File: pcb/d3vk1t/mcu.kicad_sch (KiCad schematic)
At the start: 11 parts, among them J2 Conn_01x06, U1 STM32F412RETx

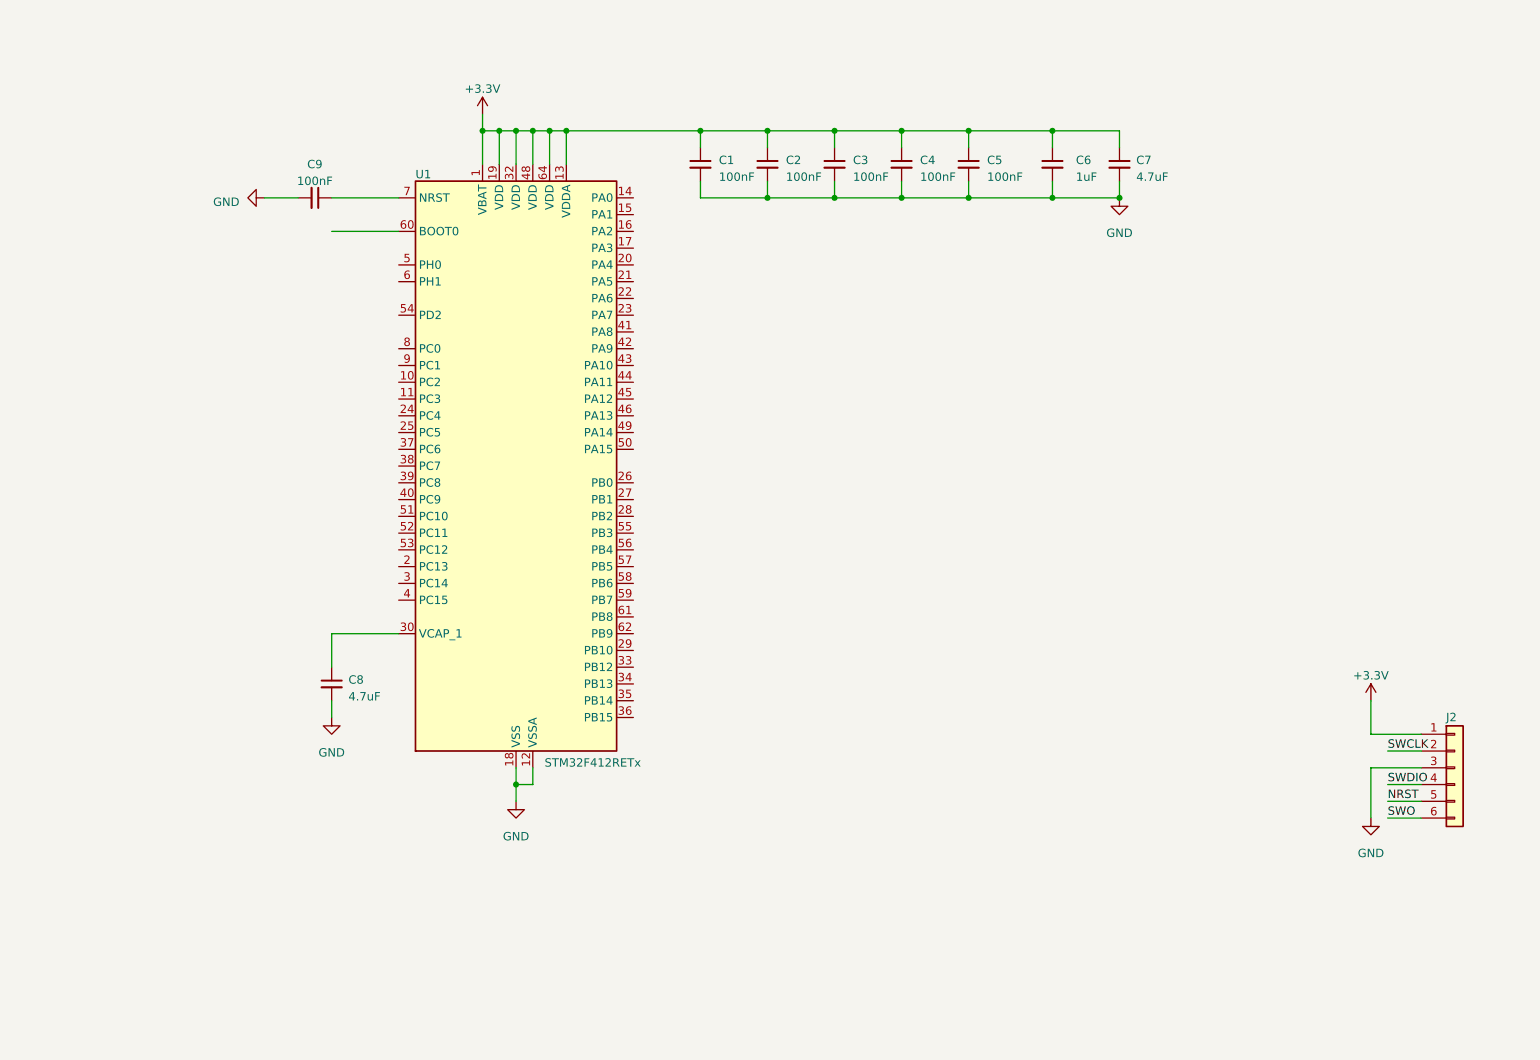
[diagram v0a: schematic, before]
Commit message: [update all schematics sheets]
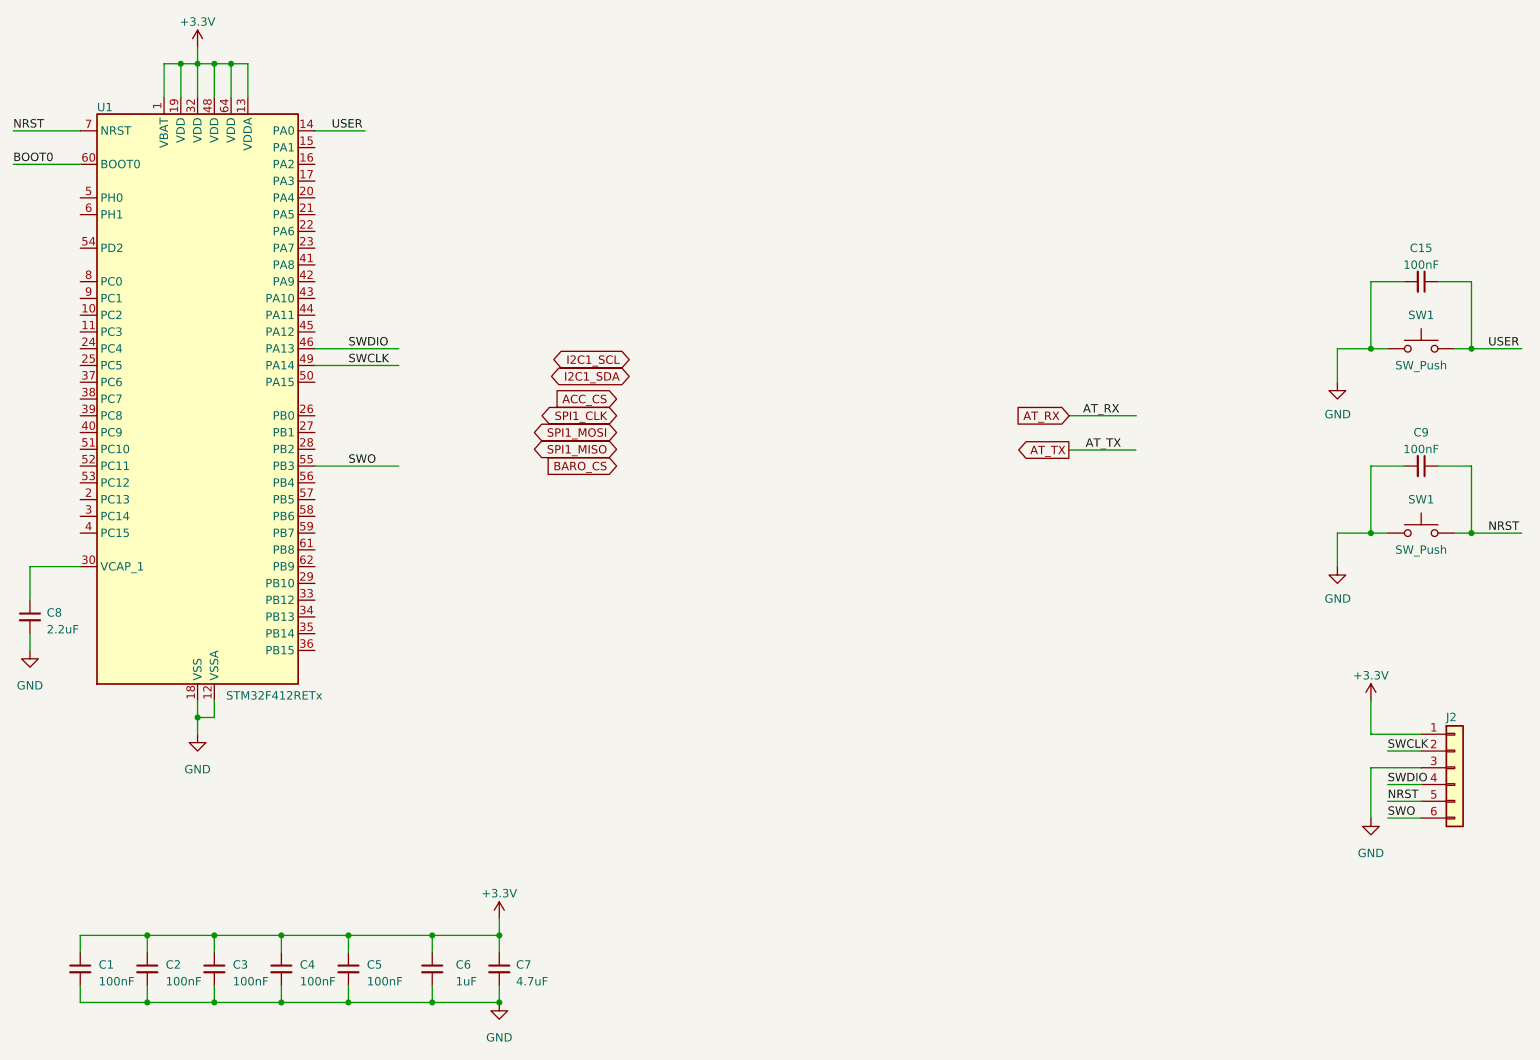
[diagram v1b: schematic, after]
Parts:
- added C15: 100nF, Capacitor_SMD:C_0402_1005Metric, symbol Device:C_Small
- added SW1 (x2): SW_Push, Button_Switch_SMD:SW_SPST_FSMSM, symbol Switch:SW_Push
- C8: value 4.7uF -> 2.2uF
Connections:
- net GND: now also C15.2, SW1.1, SW1.1
- net NRST: now also C9.1, U1.7 (NRST), SW1.2
- net SWCLK: now also U1.49 (PA14)
- net SWDIO: now also U1.46 (PA13)
- net SWO: now also U1.55 (PB3)
- net USER: now reaches U1.14 (PA0)
- net USER: now also C15.1, SW1.2
- net BOOT0: now reaches U1.60 (BOOT0)
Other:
- moved on the sheet: C1, C2, C3, C4, C5, C6, C7, C8, C9, U1
